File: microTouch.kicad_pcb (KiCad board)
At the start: 2 copper layers, 34.5 x 22.9 mm, 10 parts, among them J1 SERVO, J2 PRINTER, U1 A3144

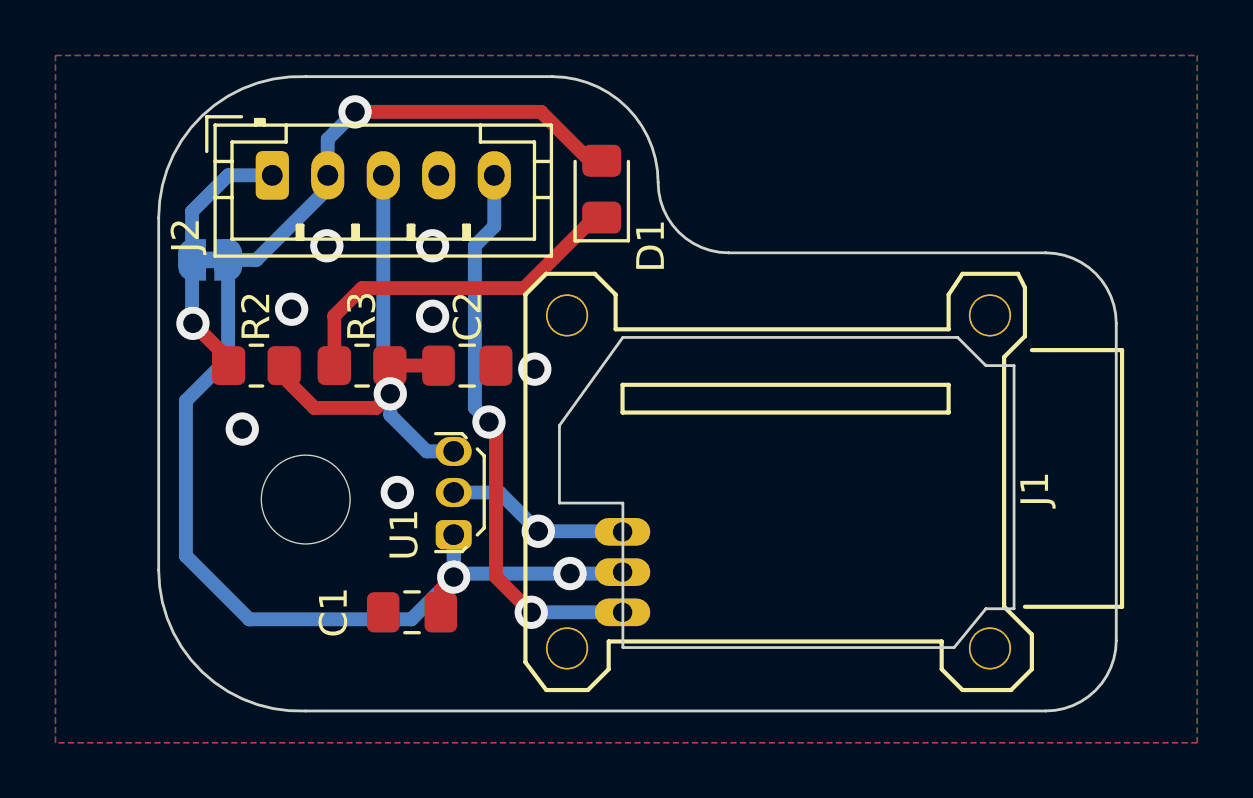
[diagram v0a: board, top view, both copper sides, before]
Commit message: a few more layout tweaks
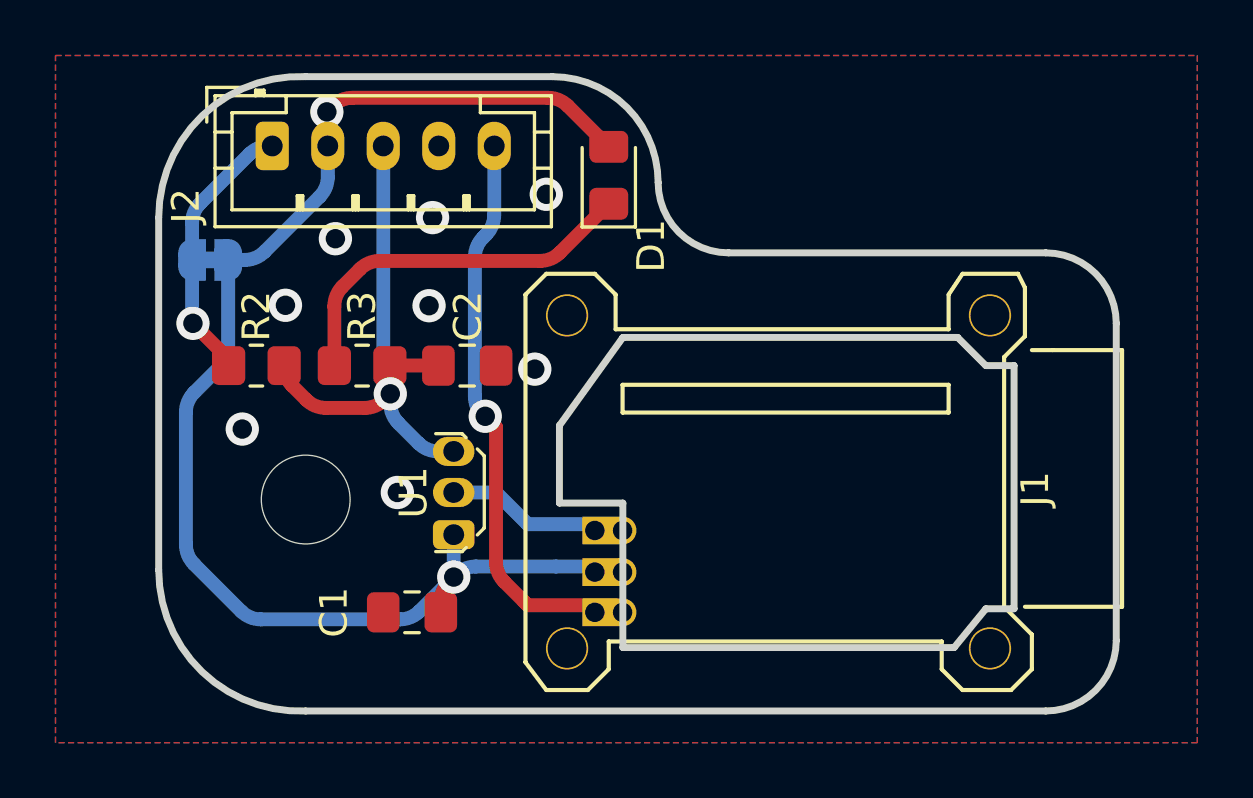
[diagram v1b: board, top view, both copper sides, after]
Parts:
- U1: footprint Package_TO_SOT_THT:TO-92Flat -> microTouch:TO-92Flat_Oval
- moved J2 1.06 mm to (99.1, 88.9)
- moved D1 0.56 mm to (111.3, 89.9)
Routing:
- net /SERVO: track 20.2 -> 21.0 mm, vias 2 -> 1
- net /SIG: track 18.2 -> 19.1 mm
- net Net-(D1-Pad1): track 12.9 -> 13.7 mm
- net /5V: track 50.5 -> 50.3 mm, vias 3 -> 2
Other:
- rule pad_to_mask_clearance: 0 -> 0.05
